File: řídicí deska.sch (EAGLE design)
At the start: 26 parts, among them IC1 MC78M12ACDTG, IC2 AZ1117CD5, Q1 NX3008, Q2 NX3008, Q3 NX3008

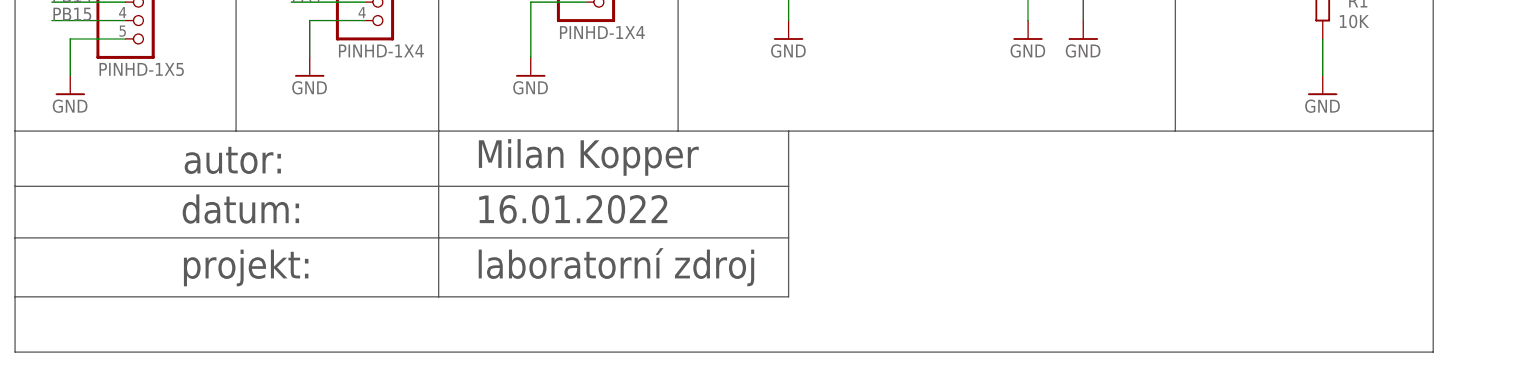
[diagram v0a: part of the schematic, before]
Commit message: doku
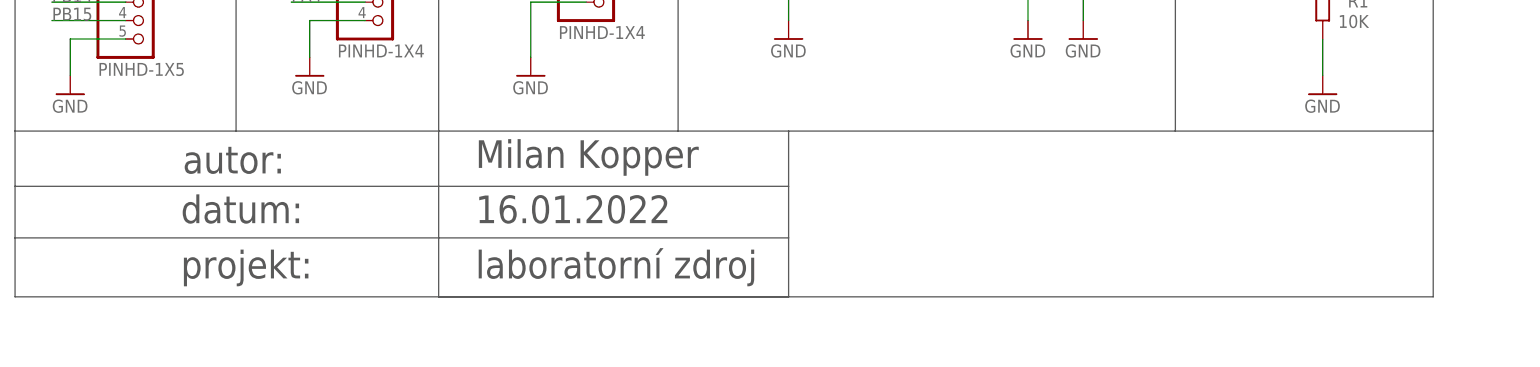
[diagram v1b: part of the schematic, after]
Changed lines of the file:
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@@
 <wire x1="0" y1="-7.62" x2="0" y2="-14.732" width="0.1524" layer="97"/>
 <wire x1="0" y1="-14.732" x2="0" y2="-22.86" width="0.1524" layer="97"/>
-<wire x1="0" y1="-22.86" x2="0" y2="-30.48" width="0.1524" layer="97"/>
-<wire x1="0" y1="-30.48" x2="195.58" y2="-30.48" width="0.1524" layer="97"/>
-<wire x1="195.58" y1="-30.48" x2="195.58" y2="0" width="0.1524" layer="97"/>
+<wire x1="58.42" y1="-22.86" x2="195.58" y2="-22.86" width="0.1524" layer="97"/>
+<wire x1="195.58" y1="-22.86" x2="195.58" y2="0" width="0.1524" layer="97"/>
 <wire x1="0" y1="215.9" x2="0" y2="236.22" width="0.1524" layer="97"/>
 <wire x1="0" y1="236.22" x2="195.58" y2="236.22" width="0.1524" layer="97"/>
